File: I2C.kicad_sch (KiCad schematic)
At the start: 12 parts, among them U13 TCA9548AMRGER

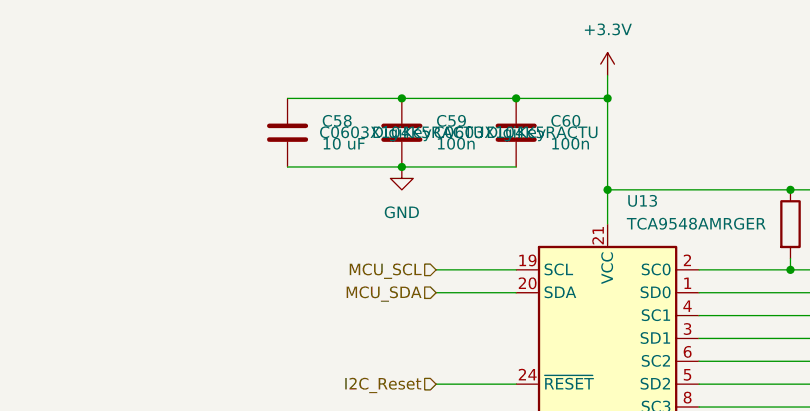
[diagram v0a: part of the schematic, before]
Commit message: Added footprints to caps
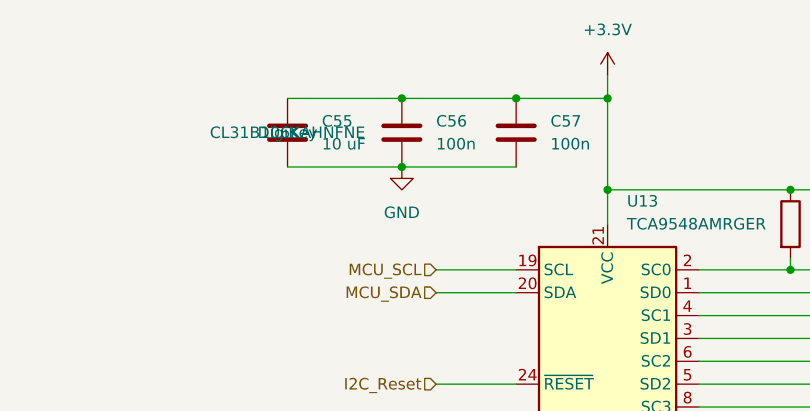
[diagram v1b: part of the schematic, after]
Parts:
- C55: renamed from C58; footprint (none) -> Capacitor_SMD:C_1206_3216Metric; MANUFACTURER (none) -> DigiKey; MANUFACTURER_PART_NUMBER (none) -> CL31B106KAHNFNE
- renumbered C59 to C56, C60 to C57
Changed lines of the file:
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@@
 		(dnp no)
 		(fields_autoplaced yes)
-		(property "Reference" "C59"
+		(property "Reference" "C56"
 			(at 110.49 54.6099 0)
 			(effects
@@
 					(size 1.27 1.27)
 				)
+				(hide yes)
 			)
 		)
@@
 					(size 1.27 1.27)
 				)
+				(hide yes)
 			)
 		)
@@
 			(project "EPS_mppt_board"
 				(path "/8f246f89-1ec7-4136-9977-839b50e116ed/0b35a7b5-b504-4fbf-9bb2-d6dcd13c2d56"
-					(reference "C59")
+					(reference "C56")
 					(unit 1)
 				)
@@
 		(dnp no)
 		(fields_autoplaced yes)
-		(property "Reference" "C58"
+		(property "Reference" "C55"
 			(at 97.79 54.6099 0)
 			(effects
@@
 			)
 		)
-		(property "Footprint" ""
+		(property "Footprint" "Capacitor_SMD:C_1206_3216Metric"
 			(at 94.9452 59.69 0)
 			(effects
@@
 			)
 		)
+		(property "MANUFACTURER" "DigiKey"
+			(at 93.98 55.88 0)
+			(effects
+				(font
+					(size 1.27 1.27)
+				)
+			)
+		)
+		(property "MANUFACTURER_PART_NUMBER" "CL31B106KAHNFNE"
+			(at 93.98 55.88 0)
+			(effects
+				(font
+					(size 1.27 1.27)
+				)
+			)
+		)
 		(pin "1"
 		)
@@
 			(project "EPS_mppt_board"
 				(path "/8f246f89-1ec7-4136-9977-839b50e116ed/0b35a7b5-b504-4fbf-9bb2-d6dcd13c2d56"
-					(reference "C58")
+					(reference "C55")
 					(unit 1)
 				)
@@
 		(dnp no)
 		(fields_autoplaced yes)
-		(property "Reference" "C60"
+		(property "Reference" "C57"
 			(at 123.19 54.6099 0)
 			(effects
@@
 					(size 1.27 1.27)
 				)
+				(hide yes)
 			)
 		)
@@
 					(size 1.27 1.27)
 				)
+				(hide yes)
 			)
 		)
@@
 			(project ""
 				(path "/8f246f89-1ec7-4136-9977-839b50e116ed/0b35a7b5-b504-4fbf-9bb2-d6dcd13c2d56"
-					(reference "C60")
-					(unit 1)
-				)
+					(reference "C57")
+					(unit 1)
+				)
